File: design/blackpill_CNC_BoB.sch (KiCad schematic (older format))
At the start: 299 parts, among them J101 ALimIN, J102 ZLimIN, J103 YLimIN, J104 XLimIN, J105 CS_IN, J106 FH_IN, J107 DoorIN, J108 ResetIN, J109 ProbeIN, J110 12V Power in, J111 AuxEncIn, J112 5V Power out, J113 ADC_in_1, J114 ADC_in_2, J115 stepDriverLim, J116 Reset, J117 UART1, J118 I2C, J119 SpindleVFD, J120 Spindle/Coolant, J121 Spindle, J122 Coolant, J123 AuxOut, J124 XStepDrv, J125 YStepDrv, J126 ZStepDrv, J127 AStepDrv, U101 TLP290-4, U102 TLP290-4, U103 TLP290-4, U104 74LVC2G17, U105 LD1117S50TR_SOT223, U106 LM358, U107 TLV9001, U108 TLV9001, U109 YAAJ_WeAct_BlackPill_Part_Like, U110 TLV9001, U111 TLV9001, U112 74HCT541, U113 74HCT541, U114 74HCT541, U115 ULN2003A, U116 ULN2003A, U117 ULN2003A

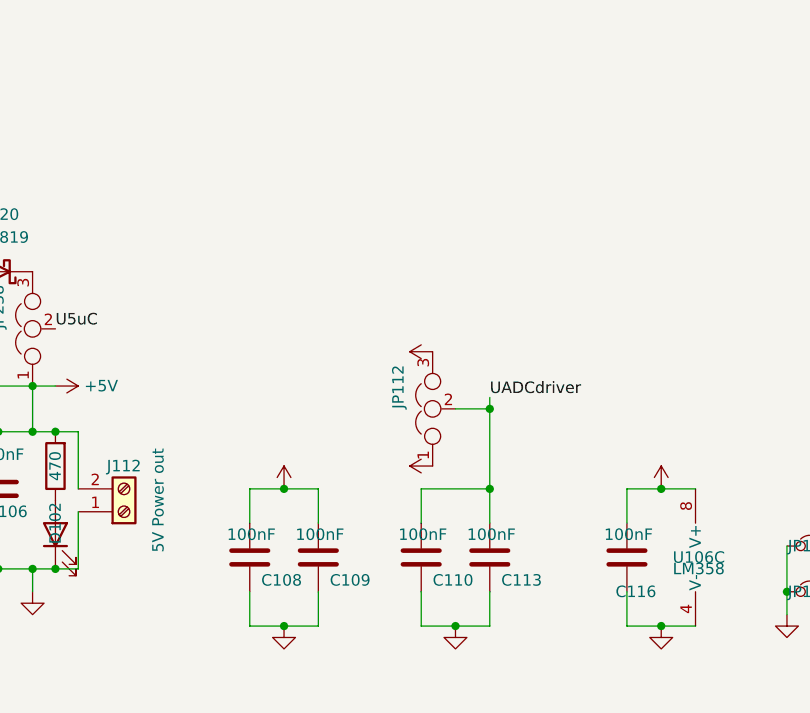
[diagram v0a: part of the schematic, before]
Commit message: place buffer cercos
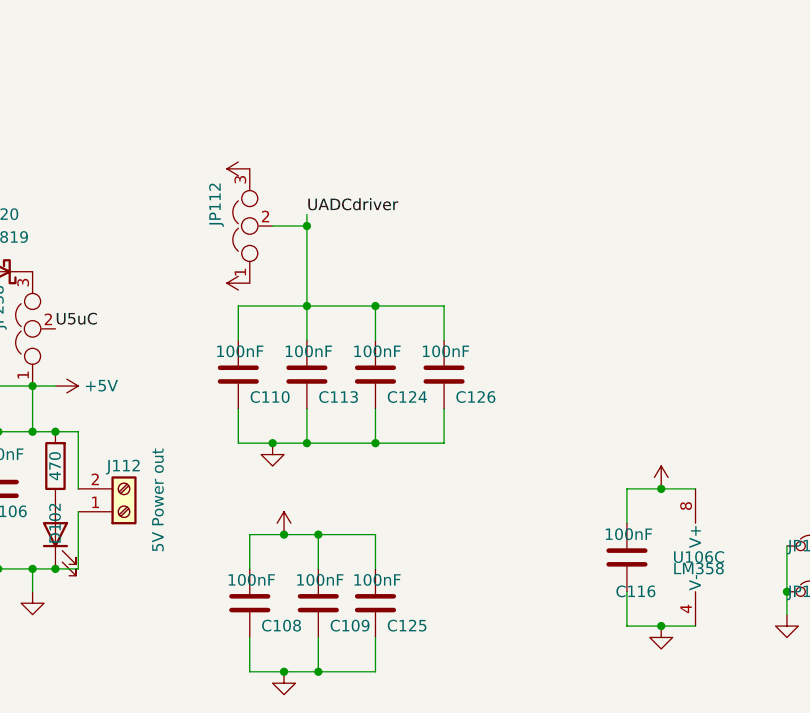
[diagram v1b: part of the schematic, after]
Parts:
- added C124, C125, C126: 100nF, Capacitor_SMD:C_0603_1608Metric, symbol Device:C
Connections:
- net +5V: now also C125.1
- net GND: now also C124.2, C125.2, C126.2
- net UADCdriver: now also C124.1, C126.1
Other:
- moved on the sheet: C108, C109, C110, C113, JP112
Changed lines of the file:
@@
-$EndComp
-$Comp
-L power:GND #PWR0118
-U 1 1 7569D2D7
-P 4700 10700
-F 0 "#PWR0118" H 4700 10450 50  0001 C CNN
-F 1 "GND" H 4750 10500 50  0001 C CNN
-F 2 "" H 4700 10700 50  0001 C CNN
-F 3 "" H 4700 10700 50  0001 C CNN
-	1    4700 10700
-	1    0    0    -1
-$EndComp
-$Comp
-L Device:C C108
-U 1 1 7569D2E3
-P 4550 10400
-F 0 "C108" H 4600 10300 50  0000 L CNN
-F 1 "100nF" H 4450 10500 50  0000 L CNN
-F 2 "Capacitor_SMD:C_0603_1608Metric" H 4588 10250 50  0001 C CNN
-F 3 "~" H 4550 10400 50  0001 C CNN
-	1    4550 10400
-	1    0    0    -1
-$EndComp
-Wire Wire Line
-	4550 10100 4550 10250
-Wire Wire Line
-	4550 10550 4550 10700
-Wire Wire Line
-	4550 10700 4700 10700
-Wire Wire Line
-	4700 10700 4850 10700
-Connection ~ 4700 10700
-$Comp
-L power:GND #PWR0127
-U 1 1 756F2E58
-P 5450 10700
-F 0 "#PWR0127" H 5450 10450 50  0001 C CNN
-F 1 "GND" H 5500 10500 50  0001 C CNN
-F 2 "" H 5450 10700 50  0001 C CNN
-F 3 "" H 5450 10700 50  0001 C CNN
-	1    5450 10700
-	1    0    0    -1
-$EndComp
-$Comp
-L Device:C C110
-U 1 1 756F2E64
-P 5300 10400
-F 0 "C110" H 5350 10300 50  0000 L CNN
-F 1 "100nF" H 5200 10500 50  0000 L CNN
-F 2 "Capacitor_SMD:C_0603_1608Metric" H 5338 10250 50  0001 C CNN
-F 3 "~" H 5300 10400 50  0001 C CNN
-	1    5300 10400
-	1    0    0    -1
-$EndComp
-Wire Wire Line
-	5300 10100 5300 10250
-Wire Wire Line
-	5300 10550 5300 10700
-Wire Wire Line
-	5300 10700 5450 10700
-Wire Wire Line
-	5450 10700 5600 10700
-Connection ~ 5450 10700
-Wire Wire Line
-	4550 10100 4700 10100
-$Comp
-L power:+5V #PWR0117
-U 1 1 73BC8B53
-P 4700 10100
-F 0 "#PWR0117" H 4700 9950 50  0001 C CNN
-F 1 "+5V" H 4750 10300 50  0001 C CNN
-F 2 "" H 4700 10100 50  0001 C CNN
-F 3 "" H 4700 10100 50  0001 C CNN
-	1    4700 10100
-	1    0    0    -1
-$EndComp
-Connection ~ 4700 10100
-Wire Wire Line
-	4700 10100 4850 10100
-$Comp
-L power:+5V #PWR0125
-U 1 1 758539CE
-P 5350 9500
-F 0 "#PWR0125" H 5350 9350 50  0001 C CNN
-F 1 "+5V" H 5400 9700 50  0001 C CNN
-F 2 "" H 5350 9500 50  0001 C CNN
-F 3 "" H 5350 9500 50  0001 C CNN
-	1    5350 9500
-	0    -1   -1   0
 $EndComp
 $Comp
@@
 Text Label 8150 4600 0    50   ~ 0
 UADCdriver
-$Comp
-L Device:C C109
-U 1 1 768A9165
-P 4850 10400
-F 0 "C109" H 4900 10300 50  0000 L CNN
-F 1 "100nF" H 4750 10500 50  0000 L CNN
-F 2 "Capacitor_SMD:C_0603_1608Metric" H 4888 10250 50  0001 C CNN
-F 3 "~" H 4850 10400 50  0001 C CNN
-	1    4850 10400
-	1    0    0    -1
-$EndComp
-$Comp
-L Device:C C113
-U 1 1 768A9343
-P 5600 10400
-F 0 "C113" H 5650 10300 50  0000 L CNN
-F 1 "100nF" H 5500 10500 50  0000 L CNN
-F 2 "Capacitor_SMD:C_0603_1608Metric" H 5638 10250 50  0001 C CNN
-F 3 "~" H 5600 10400 50  0001 C CNN
-	1    5600 10400
-	1    0    0    -1
-$EndComp
-$Comp
-L power:+3.3V #PWR0126
-U 1 1 768B85AD
-P 5350 10000
-F 0 "#PWR0126" H 5350 9850 50  0001 C CNN
-F 1 "+3.3V" H 5365 10173 50  0001 C CNN
-F 2 "" H 5350 10000 50  0001 C CNN
-F 3 "" H 5350 10000 50  0001 C CNN
-	1    5350 10000
-	0    -1   -1   0
-$EndComp
 Text Label 10700 9600 1    50   ~ 0
 UADCdriver
-Wire Wire Line
-	4850 10100 4850 10250
-Wire Wire Line
-	4850 10550 4850 10700
-Wire Wire Line
-	5600 10700 5600 10550
-Wire Wire Line
-	5600 10100 5600 10250
-$Comp
-L Device:Jumper_NC_Dual JP112
-U 1 1 76A11CC6
-P 5350 9750
-F 0 "JP112" H 5350 9900 50  0000 L CNN
-F 1 "Jumper_NC_Dual" V 5350 9900 50  0001 L CNN
-F 2 "Connector_PinHeader_2.54mm:PinHeader_1x03_P2.54mm_Vertical" H 5350 9750 50  0001 C CNN
-F 3 "~" H 5350 9750 50  0001 C CNN
-	1    5350 9750
-	0    -1   -1   0
-$EndComp
-Wire Wire Line
-	5300 10100 5600 10100
-Connection ~ 5600 10100
-Wire Wire Line
-	5600 9700 5600 9750
-Wire Wire Line
-	5450 9750 5600 9750
-Connection ~ 5600 9750
-Wire Wire Line
-	5600 9750 5600 10100
 $Comp
 L Device:R R141
@@
 Wire Wire Line
 	2900 10850 3050 10850
-Text Label 5600 9700 0    50   ~ 0
-UADCdriver
 $Comp
 L Diode:1N5819 D120
@@
 Wire Wire Line
 	6240 2980 6110 2980
+Text Label 4800 8900 0    50   ~ 0
+UADCdriver
+Wire Wire Line
+	4800 8950 4800 9300
+Connection ~ 4800 8950
+Wire Wire Line
+	4650 8950 4800 8950
+Wire Wire Line
+	4800 8900 4800 8950
+Connection ~ 4800 9300
+Wire Wire Line
+	4500 9300 4800 9300
+$Comp
+L Device:Jumper_NC_Dual JP112
+U 1 1 76A11CC6
+P 4550 8950
+F 0 "JP112" H 4550 9100 50  0000 L CNN
+F 1 "Jumper_NC_Dual" V 4550 9100 50  0001 L CNN
+F 2 "Connector_PinHeader_2.54mm:PinHeader_1x03_P2.54mm_Vertical" H 4550 8950 50  0001 C CNN
+F 3 "~" H 4550 8950 50  0001 C CNN
+	1    4550 8950
+	0    -1   -1   0
+$EndComp
+Wire Wire Line
+	4800 9300 4800 9450
+Wire Wire Line
+	4800 9900 4800 9750
+$Comp
+L power:+3.3V #PWR0126
+U 1 1 768B85AD
+P 4550 9200
+F 0 "#PWR0126" H 4550 9050 50  0001 C CNN
+F 1 "+3.3V" H 4565 9373 50  0001 C CNN
+F 2 "" H 4550 9200 50  0001 C CNN
+F 3 "" H 4550 9200 50  0001 C CNN
+	1    4550 9200
+	0    -1   -1   0
+$EndComp
+$Comp
+L Device:C C113
+U 1 1 768A9343
+P 4800 9600
+F 0 "C113" H 4850 9500 50  0000 L CNN
+F 1 "100nF" H 4700 9700 50  0000 L CNN
+F 2 "Capacitor_SMD:C_0603_1608Metric" H 4838 9450 50  0001 C CNN
+F 3 "~" H 4800 9600 50  0001 C CNN
+	1    4800 9600
+	1    0    0    -1
+$EndComp
+$Comp
+L power:+5V #PWR0125
+U 1 1 758539CE
+P 4550 8700
+F 0 "#PWR0125" H 4550 8550 50  0001 C CNN
+F 1 "+5V" H 4600 8900 50  0001 C CNN
+F 2 "" H 4550 8700 50  0001 C CNN
+F 3 "" H 4550 8700 50  0001 C CNN
+	1    4550 8700
+	0    -1   -1   0
+$EndComp
+Connection ~ 4650 9900
+Wire Wire Line
+	4650 9900 4800 9900
+Wire Wire Line
+	4500 9900 4650 9900
+Wire Wire Line
+	4500 9750 4500 9900
+Wire Wire Line
+	4500 9300 4500 9450
+$Comp
+L Device:C C110
+U 1 1 756F2E64
+P 4500 9600
+F 0 "C110" H 4550 9500 50  0000 L CNN
+F 1 "100nF" H 4400 9700 50  0000 L CNN
+F 2 "Capacitor_SMD:C_0603_1608Metric" H 4538 9450 50  0001 C CNN
+F 3 "~" H 4500 9600 50  0001 C CNN
+	1    4500 9600
+	1    0    0    -1
+$EndComp
+$Comp
+L power:GND #PWR0127
+U 1 1 756F2E58
+P 4650 9900
+F 0 "#PWR0127" H 4650 9650 50  0001 C CNN
+F 1 "GND" H 4700 9700 50  0001 C CNN
+F 2 "" H 4650 9900 50  0001 C CNN
+F 3 "" H 4650 9900 50  0001 C CNN
+	1    4650 9900
+	1    0    0    -1
+$EndComp
+Wire Wire Line
+	4850 10750 4850 10900
+Wire Wire Line
+	4850 10300 4850 10450
+$Comp
+L Device:C C109
+U 1 1 768A9165
+P 4850 10600
+F 0 "C109" H 4900 10500 50  0000 L CNN
+F 1 "100nF" H 4750 10700 50  0000 L CNN
+F 2 "Capacitor_SMD:C_0603_1608Metric" H 4888 10450 50  0001 C CNN
+F 3 "~" H 4850 10600 50  0001 C CNN
+	1    4850 10600
+	1    0    0    -1
+$EndComp
+Wire Wire Line
+	4700 10300 4850 10300
+Connection ~ 4700 10300
+$Comp
+L power:+5V #PWR0117
+U 1 1 73BC8B53
+P 4700 10300
+F 0 "#PWR0117" H 4700 10150 50  0001 C CNN
+F 1 "+5V" H 4750 10500 50  0001 C CNN
+F 2 "" H 4700 10300 50  0001 C CNN
+F 3 "" H 4700 10300 50  0001 C CNN
+	1    4700 10300
+	1    0    0    -1
+$EndComp
+Wire Wire Line
+	4550 10300 4700 10300
+Connection ~ 4700 10900
+Wire Wire Line
+	4700 10900 4850 10900
+Wire Wire Line
+	4550 10900 4700 10900
+Wire Wire Line
+	4550 10750 4550 10900
+Wire Wire Line
+	4550 10300 4550 10450
+$Comp
+L Device:C C108
+U 1 1 7569D2E3
+P 4550 10600
+F 0 "C108" H 4600 10500 50  0000 L CNN
+F 1 "100nF" H 4450 10700 50  0000 L CNN
+F 2 "Capacitor_SMD:C_0603_1608Metric" H 4588 10450 50  0001 C CNN
+F 3 "~" H 4550 10600 50  0001 C CNN
+	1    4550 10600
+	1    0    0    -1
+$EndComp
+$Comp
+L power:GND #PWR0118
+U 1 1 7569D2D7
+P 4700 10900
+F 0 "#PWR0118" H 4700 10650 50  0001 C CNN
+F 1 "GND" H 4750 10700 50  0001 C CNN
+F 2 "" H 4700 10900 50  0001 C CNN
+F 3 "" H 4700 10900 50  0001 C CNN
+	1    4700 10900
+	1    0    0    -1
+$EndComp
+$Comp
+L Device:C C125
+U 1 1 68D74ED4
+P 5100 10600
+F 0 "C125" H 5150 10500 50  0000 L CNN
+F 1 "100nF" H 5000 10700 50  0000 L CNN
+F 2 "Capacitor_SMD:C_0603_1608Metric" H 5138 10450 50  0001 C CNN
+F 3 "~" H 5100 10600 50  0001 C CNN
+	1    5100 10600
+	1    0    0    -1
+$EndComp
+$Comp
+L Device:C C124
+U 1 1 68E10737
+P 5100 9600
+F 0 "C124" H 5150 9500 50  0000 L CNN
+F 1 "100nF" H 5000 9700 50  0000 L CNN
+F 2 "Capacitor_SMD:C_0603_1608Metric" H 5138 9450 50  0001 C CNN
+F 3 "~" H 5100 9600 50  0001 C CNN
+	1    5100 9600
+	1    0    0    -1
+$EndComp
+$Comp
+L Device:C C126
+U 1 1 68E11AD2
+P 5400 9600
+F 0 "C126" H 5450 9500 50  0000 L CNN
+F 1 "100nF" H 5300 9700 50  0000 L CNN
+F 2 "Capacitor_SMD:C_0603_1608Metric" H 5438 9450 50  0001 C CNN
+F 3 "~" H 5400 9600 50  0001 C CNN
+	1    5400 9600
+	1    0    0    -1
+$EndComp
+Wire Wire Line
+	4850 10300 5100 10300
+Wire Wire Line
+	5100 10300 5100 10450
+Connection ~ 4850 10300
+Wire Wire Line
+	4850 10900 5100 10900
+Wire Wire Line
+	5100 10900 5100 10750
+Connection ~ 4850 10900
+Wire Wire Line
+	4800 9900 5100 9900
+Wire Wire Line
+	5400 9900 5400 9750
+Connection ~ 4800 9900
+Wire Wire Line
+	5100 9750 5100 9900
+Connection ~ 5100 9900
+Wire Wire Line
+	5100 9900 5400 9900
+Wire Wire Line
+	4800 9300 5100 9300
+Wire Wire Line
+	5400 9300 5400 9450
+Wire Wire Line
+	5100 9450 5100 9300
+Connection ~ 5100 9300
+Wire Wire Line
+	5100 9300 5400 9300
 $EndSCHEMATC
